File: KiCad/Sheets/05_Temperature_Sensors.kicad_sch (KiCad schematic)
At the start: 12 parts, among them U14 GAS_FLOW_SENSOR_SOCKET, U15 GAS_RETURN_SENSOR_SOCKET, U16 WOOD_FLOW_SENSOR_SOCKET, U17 WOOD_RETURN_SENSOR_SOCKET, U18 WOOD_BOILER_SENSOR_SOCKET, U4 GAS_FLOW_SENSOR, U5 GAS_RETURN_SENSOR, U6 WOOD_FLOW_SENSOR, U7 WOOD_RETURN_SENSOR, U8 WOOD_BOILER_SENSOR

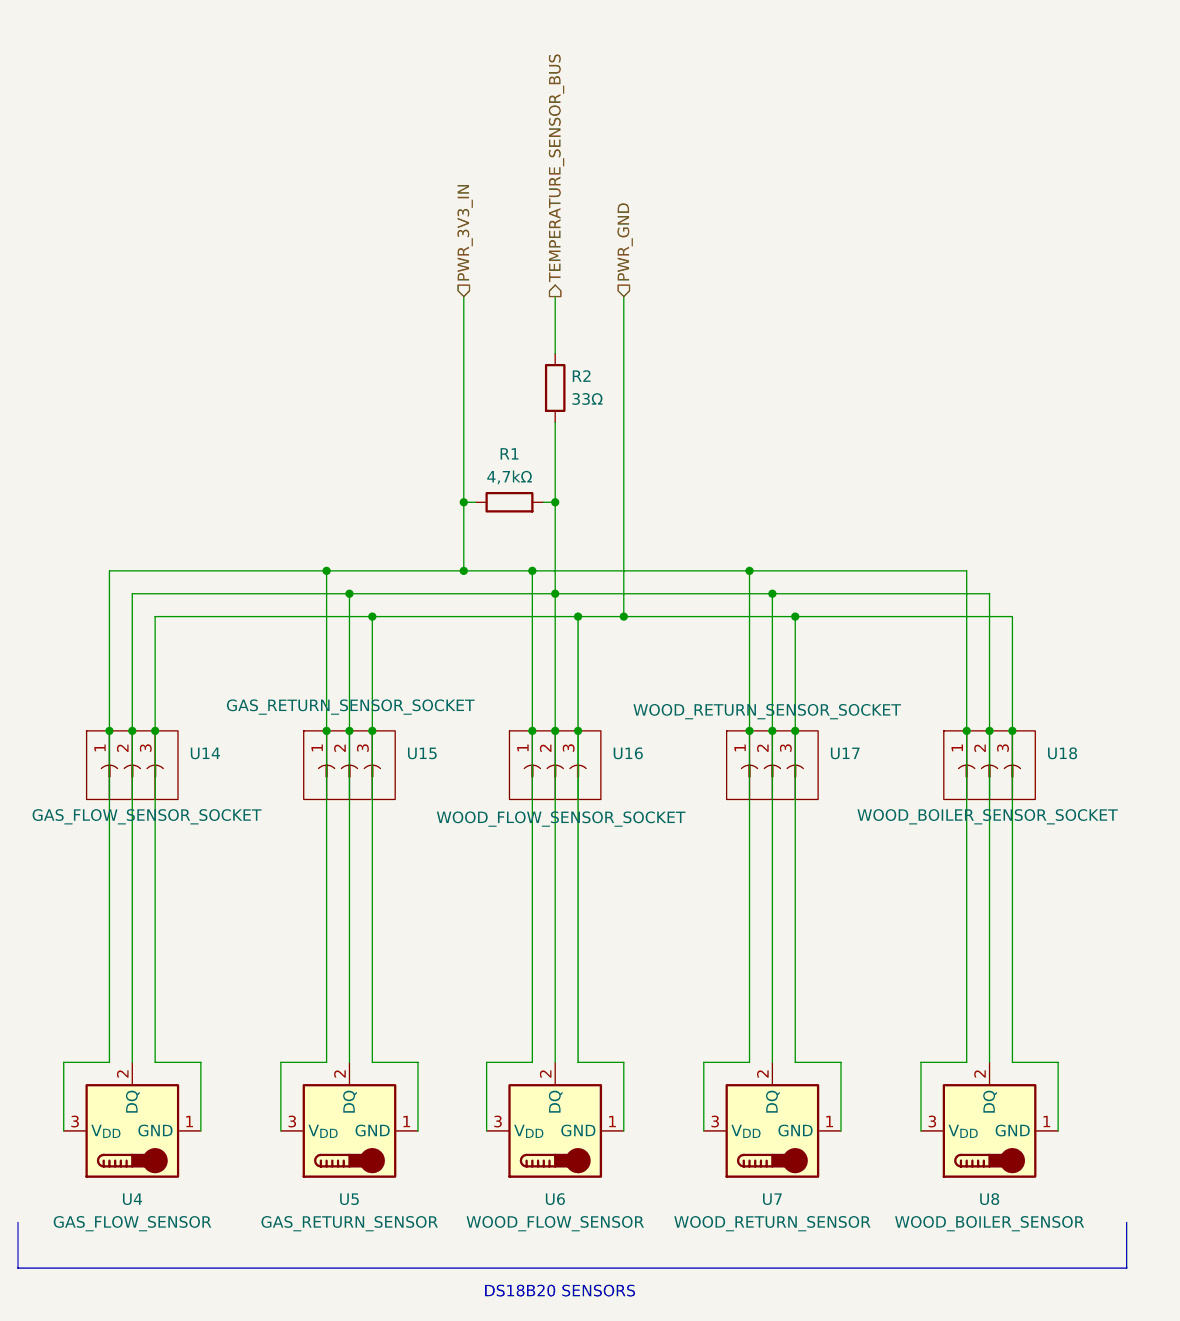
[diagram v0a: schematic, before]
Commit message: Finished PCB
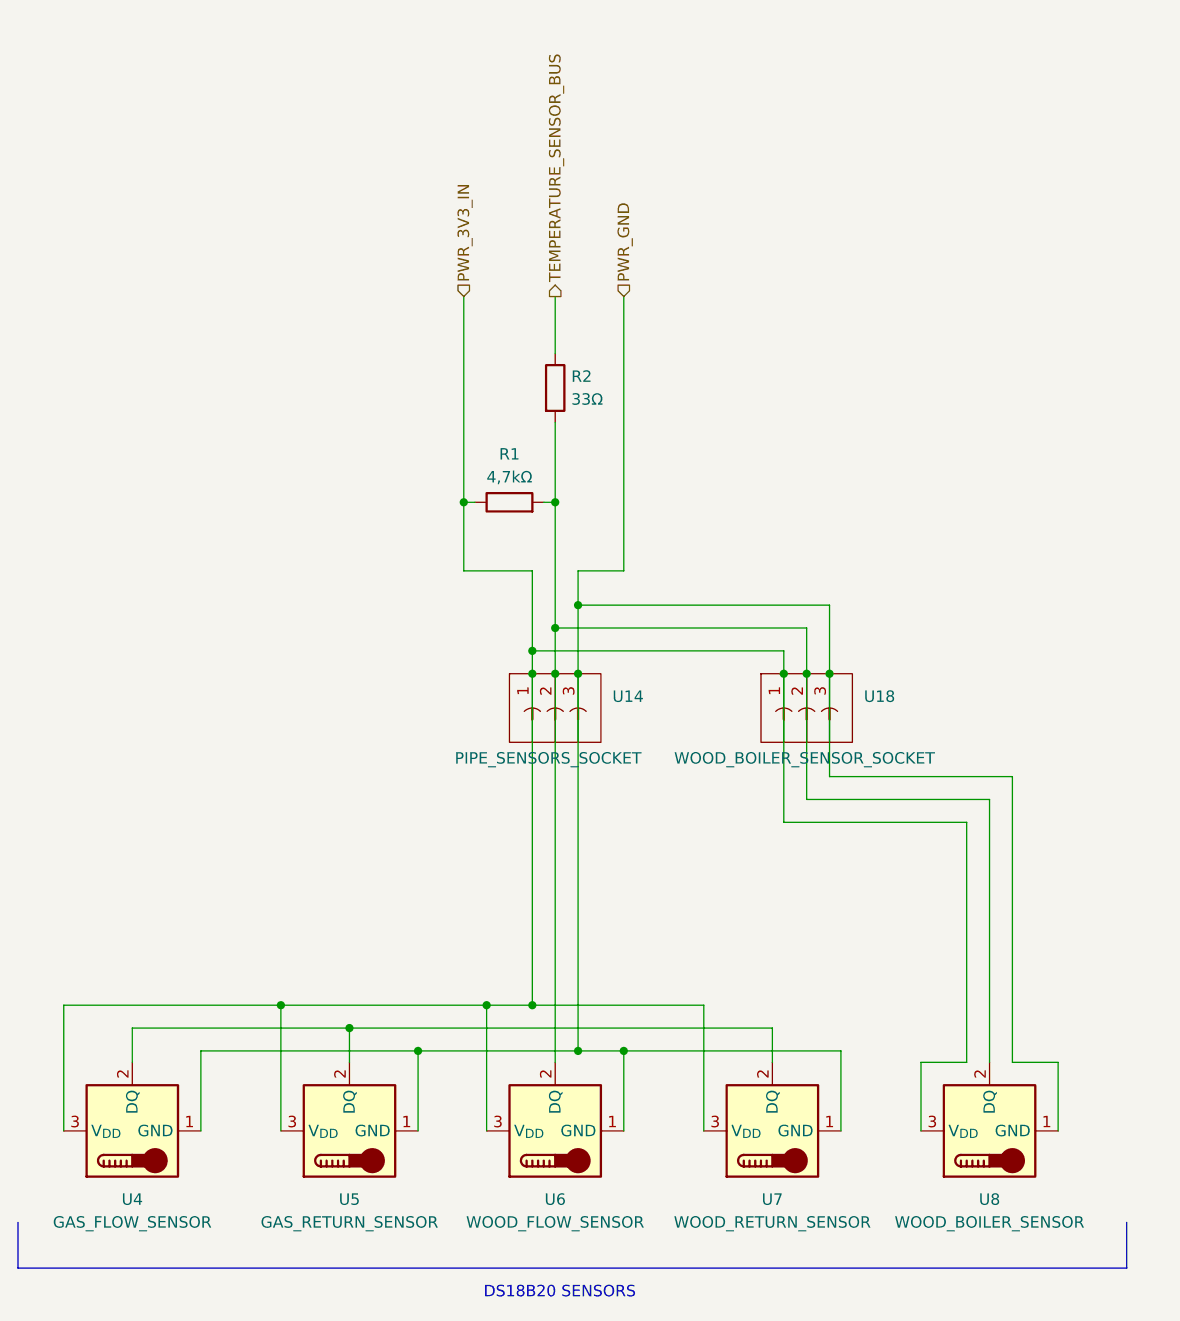
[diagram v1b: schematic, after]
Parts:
- removed U15: GAS_RETURN_SENSOR_SOCKET, Connector_JST:JST_PH_B3B-PH-K_1x03_P2.00mm_Vertical, symbol HMS_Symbols:CONN_JST_PH_3P
- removed U16: WOOD_FLOW_SENSOR_SOCKET, Connector_JST:JST_PH_B3B-PH-K_1x03_P2.00mm_Vertical, symbol HMS_Symbols:CONN_JST_PH_3P
- removed U17: WOOD_RETURN_SENSOR_SOCKET, Connector_JST:JST_PH_B3B-PH-K_1x03_P2.00mm_Vertical, symbol HMS_Symbols:CONN_JST_PH_3P
- U14: value GAS_FLOW_SENSOR_SOCKET -> PIPE_SENSORS_SOCKET; footprint Connector_JST:JST_PH_B3B-PH-K_1x03_P2.00mm_Vertical -> Connector_JST:JST_XH_B3B-XH-A_1x03_P2.50mm_Vertical
- U18: footprint Connector_JST:JST_PH_B3B-PH-K_1x03_P2.00mm_Vertical -> Connector_JST:JST_XH_B3B-XH-A_1x03_P2.50mm_Vertical
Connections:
- net at R1.2, R2.2, U14.2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: no longer U4.2 (DQ), U5.2 (DQ), U7.2 (DQ)
- new net: U4.2 (DQ), U5.2 (DQ), U7.2 (DQ)
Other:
- moved on the sheet: U14, U18
